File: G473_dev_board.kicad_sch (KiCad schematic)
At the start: 44 parts, among them J2 Conn_01x04_Pin, J3 Conn_01x04_Pin, J4 Conn_01x02_Pin, Q15 MMBTA06, SW1 SW_Push, SW2 SW_Push, U1 STM32G473VETx, U17 24LC512-E/SN, Y1 ECS-3225MVLC-080-CN-TR, Y2 ECS-327ATQMV-AS-TR

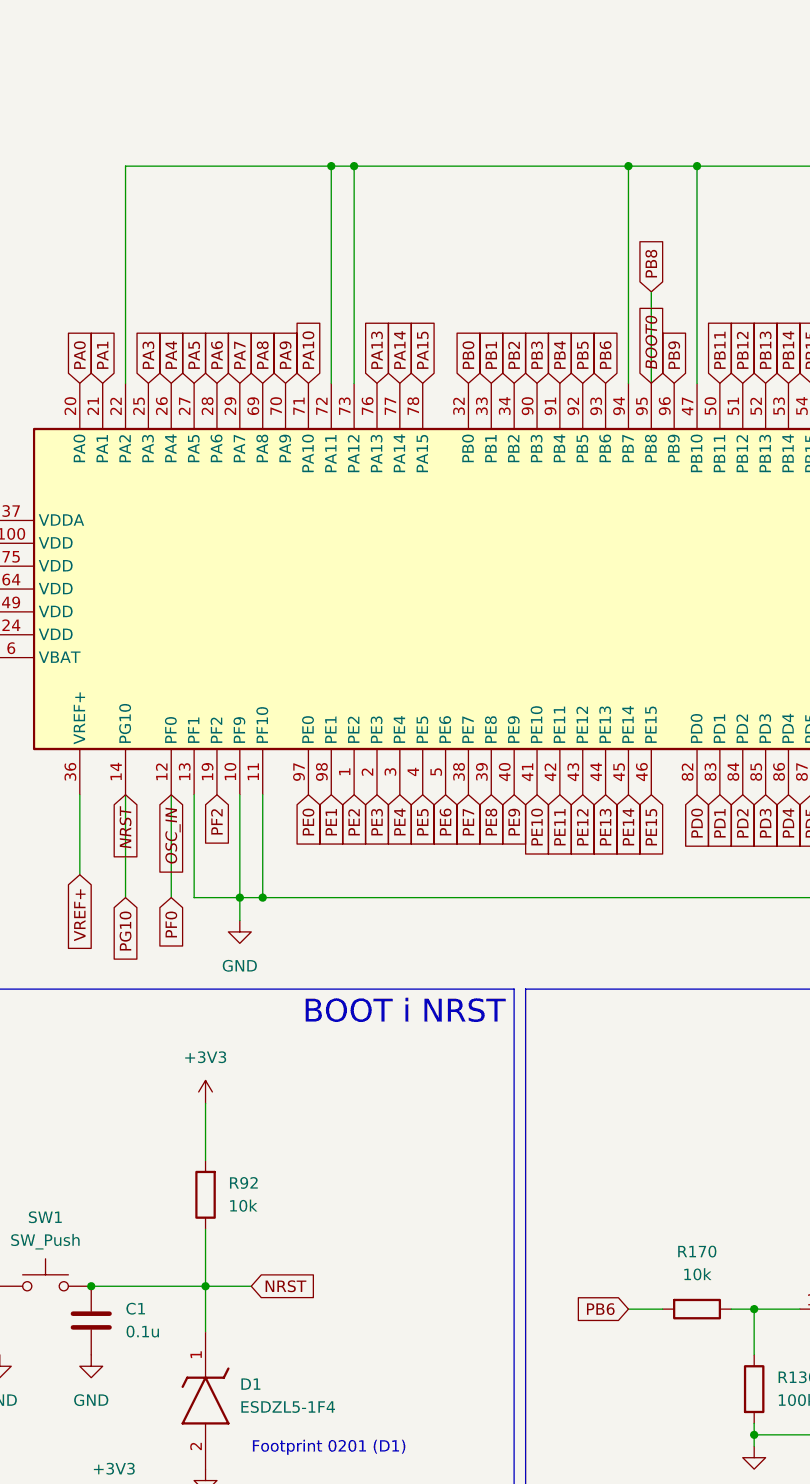
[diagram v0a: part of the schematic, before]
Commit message: Zaktualizowano pliki
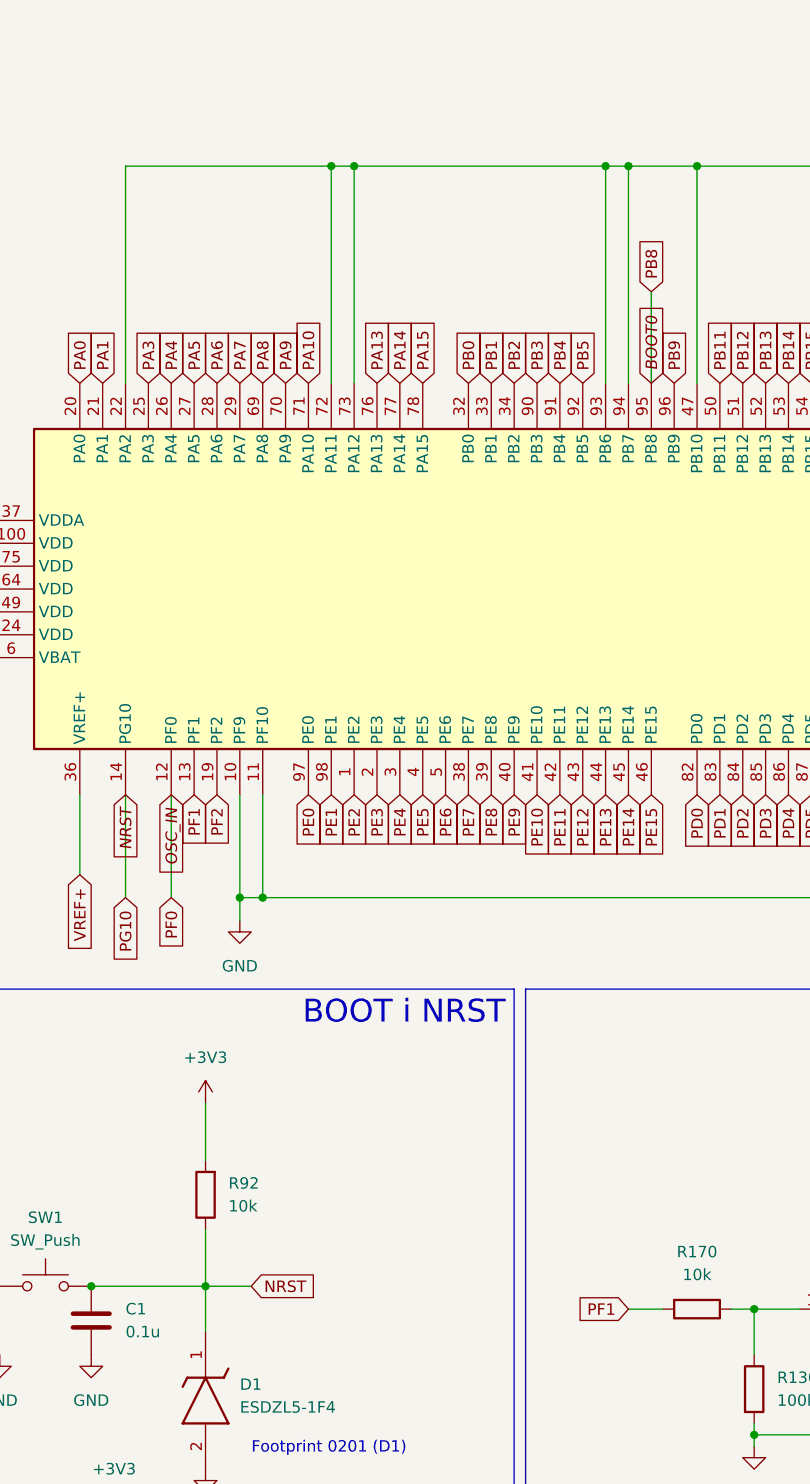
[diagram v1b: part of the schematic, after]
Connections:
- net GND: now also U1.93 (PB6); no longer U1.13 (PF1)
- net PB6 renamed PF1
- net PF1: now also U1.13 (PF1); no longer U1.93 (PB6)
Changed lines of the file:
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@@
 	)
 	(junction
+		(at 106.68 19.05)
+		(diameter 0)
+		(color 0 0 0 0)
+	)
+	(junction
 		(at 116.84 19.05)
 		(diameter 0)
@@
 	(wire
 		(pts
-			(xy 78.74 19.05) (xy 109.22 19.05)
+			(xy 78.74 19.05) (xy 106.68 19.05)
 		)
 		(stroke
@@
 	(wire
 		(pts
-			(xy 60.96 88.9) (xy 60.96 100.33)
-		)
-		(stroke
-			(width 0)
-			(type default)
-		)
-	)
-	(wire
-		(pts
 			(xy 303.53 72.39) (xy 303.53 73.66)
 		)
@@
 	(wire
 		(pts
-			(xy 66.04 100.33) (xy 60.96 100.33)
-		)
-		(stroke
-			(width 0)
-			(type default)
-		)
-	)
-	(wire
-		(pts
 			(xy 179.07 185.42) (xy 185.42 185.42)
 		)
@@
 	(wire
 		(pts
+			(xy 106.68 19.05) (xy 109.22 19.05)
+		)
+		(stroke
+			(width 0)
+			(type default)
+		)
+	)
+	(wire
+		(pts
 			(xy 229.87 176.53) (xy 212.09 176.53)
 		)
@@
 	(wire
 		(pts
+			(xy 106.68 19.05) (xy 106.68 43.18)
+		)
+		(stroke
+			(width 0)
+			(type default)
+		)
+	)
+	(wire
+		(pts
 			(xy 109.22 146.05) (xy 113.03 146.05)
 		)
@@
 		)
 	)
-	(global_label "PB6"
-		(shape input)
-		(at 109.22 146.05 180)
-		(fields_autoplaced yes)
-		(effects
-			(font
-				(size 1.27 1.27)
-			)
-			(justify right)
-		)
-		(property "Intersheetrefs" "${INTERSHEET_REFS}"
-			(at 102.4853 146.05 0)
-			(effects
-				(font
-					(size 1.27 1.27)
-				)
-				(justify right)
-				(hide yes)
-			)
-		)
-	)
 	(global_label "PC8"
 		(shape input)
@@
 		)
 	)
+	(global_label "PF1"
+		(shape input)
+		(at 109.22 146.05 180)
+		(fields_autoplaced yes)
+		(effects
+			(font
+				(size 1.27 1.27)
+			)
+			(justify right)
+		)
+		(property "Intersheetrefs" "${INTERSHEET_REFS}"
+			(at 102.6667 146.05 0)
+			(effects
+				(font
+					(size 1.27 1.27)
+				)
+				(justify right)
+				(hide yes)
+			)
+		)
+	)
 	(global_label "PD15"
 		(shape input)
@@
 		)
 	)
-	(global_label "PB6"
-		(shape input)
-		(at 106.68 43.18 90)
-		(fields_autoplaced yes)
-		(effects
-			(font
-				(size 1.27 1.27)
-			)
-			(justify left)
-		)
-		(property "Intersheetrefs" "${INTERSHEET_REFS}"
-			(at 106.68 36.4453 90)
-			(effects
-				(font
-					(size 1.27 1.27)
-				)
-				(justify left)
-				(hide yes)
-			)
-		)
-	)
 	(global_label "PE14"
 		(shape input)
@@
 				(hide yes)
 			)
+		)
+	)
+	(global_label "PF1"
+		(shape input)
+		(at 60.96 88.9 270)
+		(fields_autoplaced yes)
+		(effects
+			(font
+				(size 1.27 1.27)
+			)
+			(justify right)
+		)
+		(property "Intersheetrefs" "${INTERSHEET_REFS}"
+			(at 60.96 95.4533 90)
+			(effects
+				(font
+					(size 1.27 1.27)
+				)
+				(justify right)
+				(hide yes)
+			)
